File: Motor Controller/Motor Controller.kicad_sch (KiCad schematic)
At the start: 5 parts, among them J1 Conn_01x03_Pin, U1 SN74LV1T34DBV

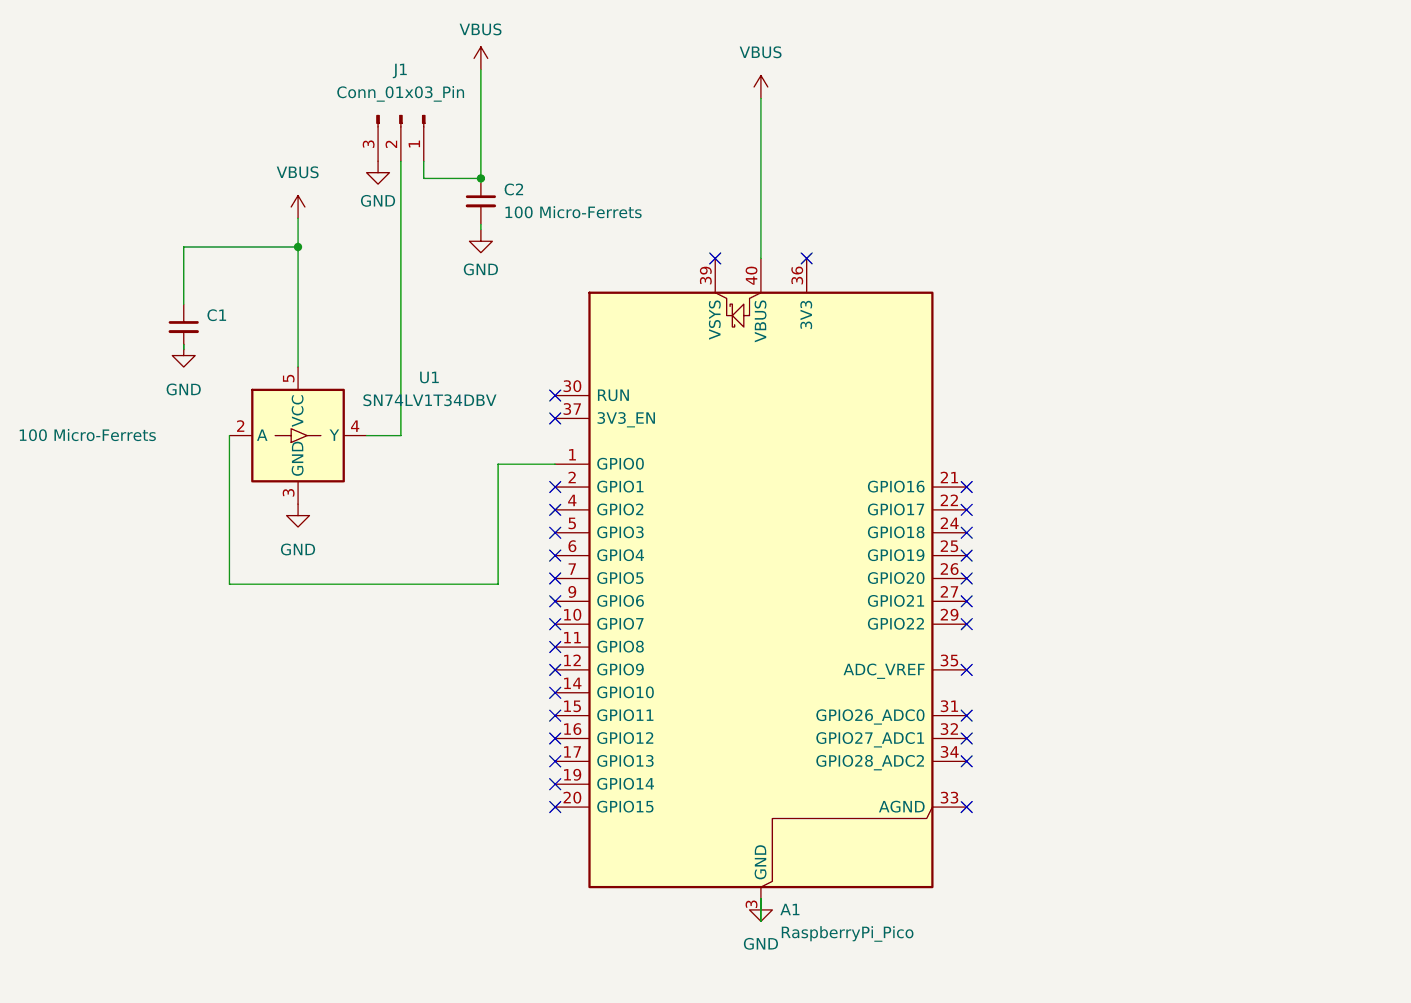
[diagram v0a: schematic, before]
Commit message: fixed grid measurements and organization q-q
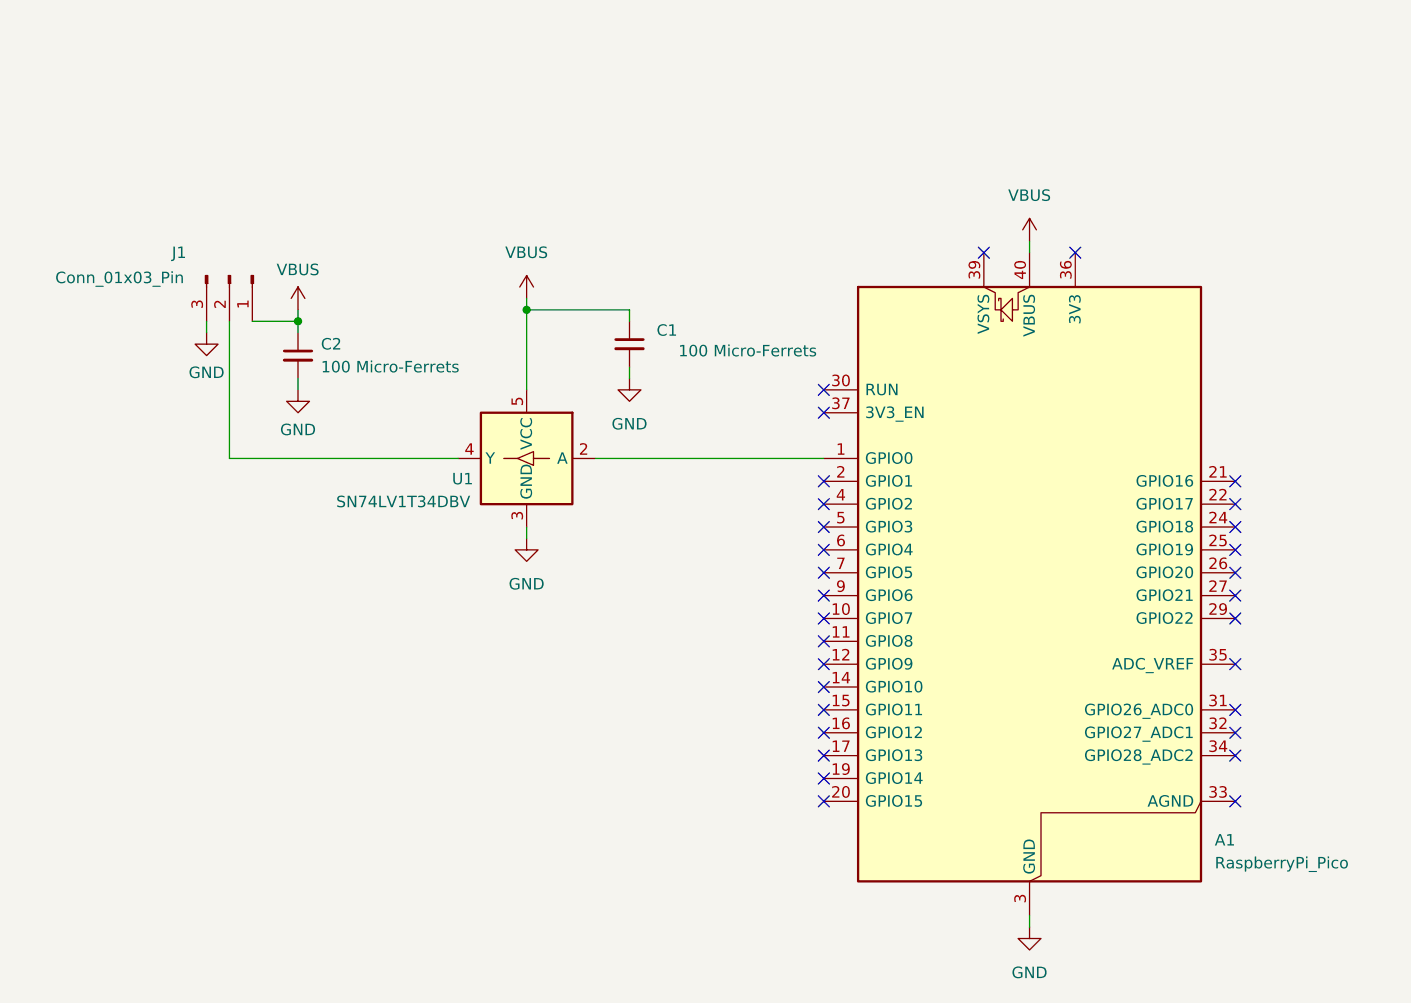
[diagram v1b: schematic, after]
